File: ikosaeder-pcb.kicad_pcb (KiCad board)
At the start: 2 copper layers, 21.9 x 20.8 mm, 7 parts

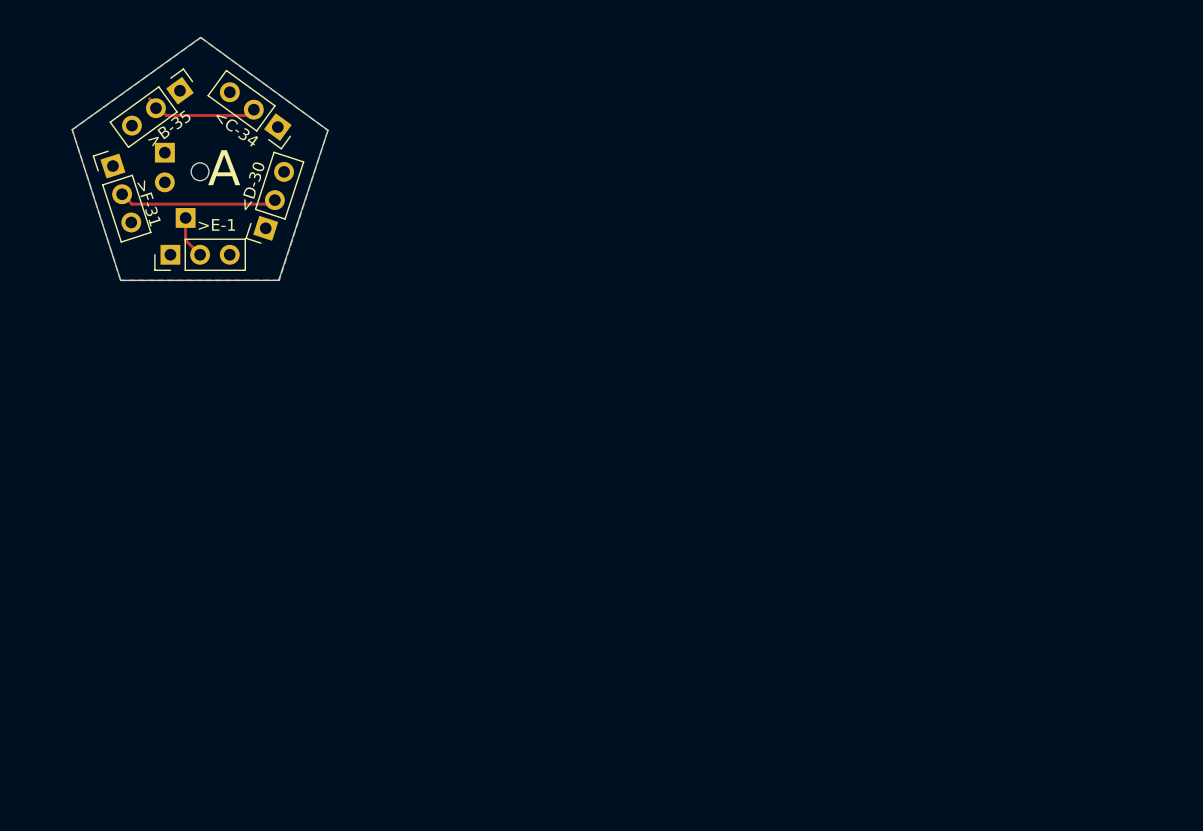
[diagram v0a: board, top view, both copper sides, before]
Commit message: Ikosaeder final
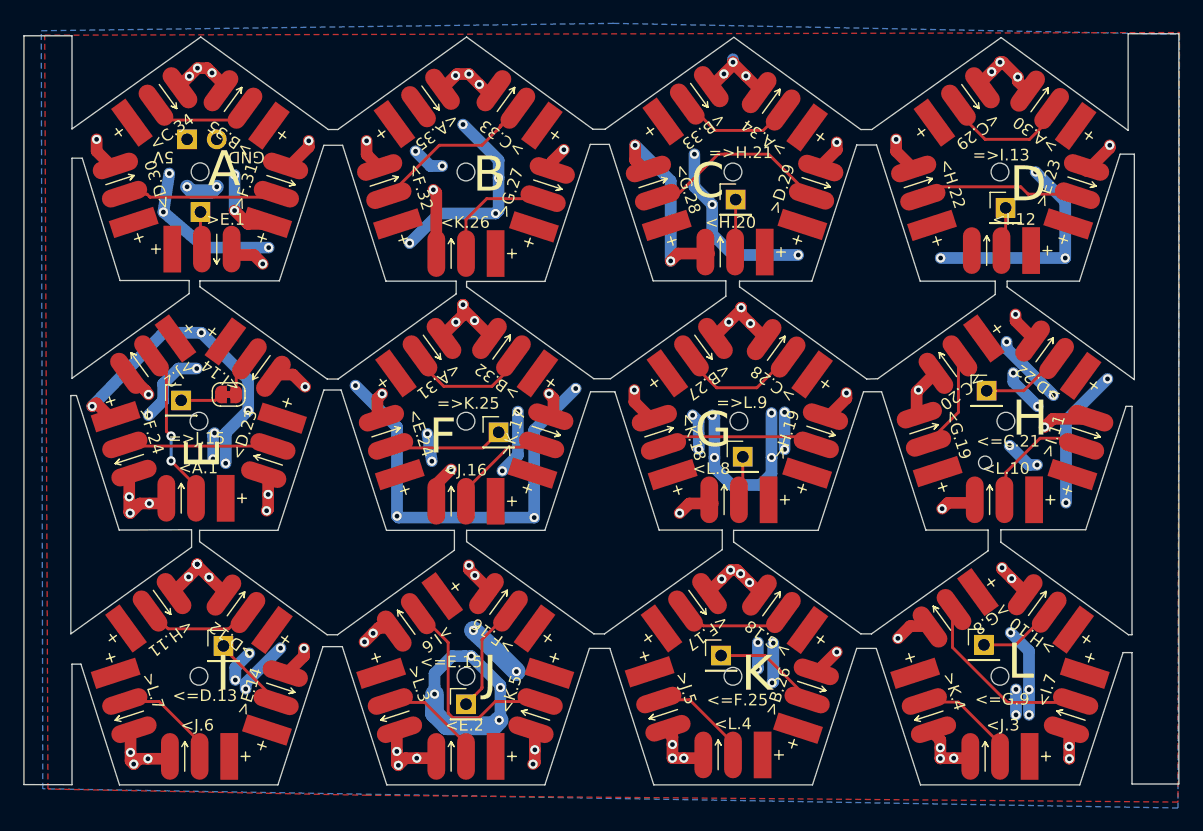
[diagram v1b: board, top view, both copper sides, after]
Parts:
- removed <C-34, <D-30: Conn_01x03_Female, Connector_PinSocket_2.54mm:PinSocket_1x03_P2.54mm_Vertical
- removed >B-35, >E-1, >F-31: Conn_01x03_Male, Connector_PinHeader_2.54mm:PinHeader_1x03_P2.54mm_Vertical
- added <=C.21: Conn_01x01_Female, Connector_PinHeader_2.54mm:PinHeader_1x01_P2.54mm_Vertical, F.Cu at (174.1, 105.6)
- added <=D.13: Conn_01x01_Female, Connector_PinHeader_2.54mm:PinHeader_1x01_P2.54mm_Vertical, F.Cu at (108.8, 127.4)
- added <=E.15: Conn_01x01_Female, Connector_PinHeader_2.54mm:PinHeader_1x01_P2.54mm_Vertical, F.Cu at (129.5, 132.4)
- added <=F.25: Conn_01x01_Female, Connector_PinHeader_2.54mm:PinHeader_1x01_P2.54mm_Vertical, F.Cu at (151.4, 128.3)
- added <=G.9: Conn_01x01_Female, Connector_PinHeader_2.54mm:PinHeader_1x01_P2.54mm_Vertical, F.Cu at (173.9, 127.4)
- added <A.1: LEDs_In, IkosaederFootprints:LED-Strip, F.Cu at (106.4, 114.8)
- added <A.31: LEDs_In, IkosaederFootprints:LED-Strip, F.Cu at (125.6, 102.6)
- added <A.35: LEDs_In, IkosaederFootprints:LED-Strip, F.Cu at (125.5, 81.3)
- added <B.27: LEDs_In, IkosaederFootprints:LED-Strip, F.Cu at (148.8, 102.6)
- added <B.33: LEDs_In, IkosaederFootprints:LED-Strip, F.Cu at (148.5, 81.1)
- added <C.29: LEDs_In, IkosaederFootprints:LED-Strip, F.Cu at (171.7, 81.2)
- added <C.34: LEDs_In, IkosaederFootprints:LED-Strip, F.Cu at (103.0, 81.2)
- added <D.23: LEDs_In, IkosaederFootprints:LED-Strip, F.Cu at (113.0, 110.4)
- added <D.30: LEDs_In, IkosaederFootprints:LED-Strip, F.Cu at (100.3, 88.8)
- added <E.2: LEDs_In, IkosaederFootprints:LED-Strip, F.Cu at (129.5, 136.9)
- added <E.24: LEDs_In, IkosaederFootprints:LED-Strip, F.Cu at (123.1, 110.4)
- added <F.17: LEDs_In, IkosaederFootprints:LED-Strip, F.Cu at (148.3, 124.5)
- added <F.32: LEDs_In, IkosaederFootprints:LED-Strip, F.Cu at (122.9, 88.9)
- added <G.19: LEDs_In, IkosaederFootprints:LED-Strip, F.Cu at (169.1, 110.1)
- added <G.28: LEDs_In, IkosaederFootprints:LED-Strip, F.Cu at (145.9, 89.0)
- added <H.11: LEDs_In, IkosaederFootprints:LED-Strip, F.Cu at (102.5, 124.5)
- added <H.20: LEDs_In, IkosaederFootprints:LED-Strip, F.Cu at (152.6, 93.7)
- added <H.22: LEDs_In, IkosaederFootprints:LED-Strip, F.Cu at (168.7, 89.0)
- added <I.12: LEDs_In, IkosaederFootprints:LED-Strip, F.Cu at (175.4, 93.6)
- added <I.14: LEDs_In, IkosaederFootprints:LED-Strip, F.Cu at (111.0, 102.9)
- added <I.7: LEDs_In, IkosaederFootprints:LED-Strip, F.Cu at (181.7, 132.2)
- added <J.16: LEDs_In, IkosaederFootprints:LED-Strip, F.Cu at (129.5, 115.1)
- added <J.3: LEDs_In, IkosaederFootprints:LED-Strip, F.Cu at (175.3, 136.9)
- added <J.6: LEDs_In, IkosaederFootprints:LED-Strip, F.Cu at (106.7, 136.9)
- added <K.18: LEDs_In, IkosaederFootprints:LED-Strip, F.Cu at (146.5, 110.4)
- added <K.26: LEDs_In, IkosaederFootprints:LED-Strip, F.Cu at (129.5, 93.9)
- added <K.5: LEDs_In, IkosaederFootprints:LED-Strip, F.Cu at (135.9, 132.2)
- added <L.10: LEDs_In, IkosaederFootprints:LED-Strip, F.Cu at (175.6, 114.9)
- added <L.4: LEDs_In, IkosaederFootprints:LED-Strip, F.Cu at (152.4, 136.8)
- added <L.8: LEDs_In, IkosaederFootprints:LED-Strip, F.Cu at (152.9, 114.9)
- added =>H.21: Conn_01x01_Male, Connector_PinHeader_2.54mm:PinHeader_1x01_P2.54mm_Vertical, F.Cu at (152.6, 89.2)
- added =>I.13: Conn_01x01_Male, Connector_PinHeader_2.54mm:PinHeader_1x01_P2.54mm_Vertical, F.Cu at (175.7, 89.9)
- added =>J.15: Conn_01x01_Male, Connector_PinHeader_2.54mm:PinHeader_1x01_P2.54mm_Vertical, F.Cu at (105.2, 106.4)
- added =>K.25: Conn_01x01_Male, Connector_PinHeader_2.54mm:PinHeader_1x01_P2.54mm_Vertical, F.Cu at (132.3, 109.2)
- added =>L.9: Conn_01x01_Male, Connector_PinHeader_2.54mm:PinHeader_1x01_P2.54mm_Vertical, F.Cu at (153.2, 111.3)
- added >A.30: LEDs_Out, IkosaederFootprints:LED-Strip, F.Cu at (179.7, 81.4)
- added >A.34: LEDs_Out, IkosaederFootprints:LED-Strip, F.Cu at (156.7, 81.6)
- added >B.26: LEDs_Out, IkosaederFootprints:LED-Strip, F.Cu at (158.8, 132.1)
- added >B.32: LEDs_Out, IkosaederFootprints:LED-Strip, F.Cu at (133.6, 102.6)
- added >B.35: LEDs_Out, IkosaederFootprints:LED-Strip, F.Cu at (110.6, 81.4)
- added >C.20: LEDs_Out, IkosaederFootprints:LED-Strip, F.Cu at (171.8, 102.6)
- added >C.28: LEDs_Out, IkosaederFootprints:LED-Strip, F.Cu at (157.1, 102.7)
- added >C.33: LEDs_Out, IkosaederFootprints:LED-Strip, F.Cu at (134.0, 81.4)
- added >D.12: LEDs_Out, IkosaederFootprints:LED-Strip, F.Cu at (110.9, 124.6)
- added >D.22: LEDs_Out, IkosaederFootprints:LED-Strip, F.Cu at (180.1, 102.8)
- added >D.29: LEDs_Out, IkosaederFootprints:LED-Strip, F.Cu at (159.1, 88.9)
- added >E.1: LEDs_Out, IkosaederFootprints:LED-Strip, F.Cu at (106.9, 93.5)
- added >E.14: LEDs_Out, IkosaederFootprints:LED-Strip, F.Cu at (113.3, 132.2)
- added >E.23: LEDs_Out, IkosaederFootprints:LED-Strip, F.Cu at (181.9, 88.9)
- added >F.16: LEDs_Out, IkosaederFootprints:LED-Strip, F.Cu at (133.3, 124.5)
- added >F.24: LEDs_Out, IkosaederFootprints:LED-Strip, F.Cu at (100.3, 110.2)
- added >F.31: LEDs_Out, IkosaederFootprints:LED-Strip, F.Cu at (113.3, 88.8)
- added >G.18: LEDs_Out, IkosaederFootprints:LED-Strip, F.Cu at (156.7, 124.6)
- added >G.27: LEDs_Out, IkosaederFootprints:LED-Strip, F.Cu at (136.1, 89.2)
- added >G.8: LEDs_Out, IkosaederFootprints:LED-Strip, F.Cu at (171.3, 124.3)
- added >H.10: LEDs_Out, IkosaederFootprints:LED-Strip, F.Cu at (179.5, 124.6)
- added >H.19: LEDs_Out, IkosaederFootprints:LED-Strip, F.Cu at (159.5, 110.2)
- added >I.11: LEDs_Out, IkosaederFootprints:LED-Strip, F.Cu at (182.2, 110.4)
- added >I.6: LEDs_Out, IkosaederFootprints:LED-Strip, F.Cu at (125.5, 124.7)
- added >J.2: LEDs_Out, IkosaederFootprints:LED-Strip, F.Cu at (102.6, 102.6)
- added >J.5: LEDs_Out, IkosaederFootprints:LED-Strip, F.Cu at (146.1, 132.1)
- added >K.17: LEDs_Out, IkosaederFootprints:LED-Strip, F.Cu at (136.0, 110.2)
- added >K.4: LEDs_Out, IkosaederFootprints:LED-Strip, F.Cu at (168.8, 132.2)
- added >L.3: LEDs_Out, IkosaederFootprints:LED-Strip, F.Cu at (123.1, 132.2)
- added >L.7: LEDs_Out, IkosaederFootprints:LED-Strip, F.Cu at (100.3, 132.2)
- added G***: LOGO, LOGO, B.Cu at (175.3, 123.9)
- added G***: LOGO, LOGO, B.Cu at (152.4, 87.1)
- added G***: LOGO, LOGO, B.Cu at (132.8, 91.9)
- added G***: LOGO, LOGO, B.Cu at (152.5, 130.2)
- added G***: LOGO, LOGO, B.Cu at (135.4, 128.2)
- added G***: LOGO, LOGO, B.Cu at (106.7, 124.0)
- added G***: LOGO, LOGO, B.Cu at (110.3, 113.4)
- added G***: LOGO, LOGO, B.Cu at (125.8, 113.8)
- added G***: LOGO, LOGO, B.Cu at (153.1, 102.0)
- added G***: LOGO, LOGO, B.Cu at (170.0, 106.5)
- added G***: LOGO, LOGO, B.Cu at (179.4, 92.3)
- added JP1: SolderJumper_2_Bridged, Jumper:SolderJumper-2_P1.3mm_Bridged_RoundedPad1.0x1.5mm, F.Cu at (109.2, 105.9)
- moved Power1 2.22 mm to (105.7, 84.1), turned to -90 degrees
- moved DIN1 1.37 mm to (106.8, 90.3)
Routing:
- net +5V: track 0.00 -> 254.8 mm, vias 0 -> 70
- net GND: track 0.00 -> 190.5 mm, vias 0 -> 79
- net Net-(<K.5-Pad2): track 0.00 -> 18.9 mm
- net Net-(<G.28-Pad2): track 0.00 -> 16.5 mm
- net Net-(<I.7-Pad2): track 0.00 -> 16.0 mm
- net Net-(<F.32-Pad2): track 0.00 -> 16.0 mm
- net Net-(<D.30-Pad2): track 0.00 -> 15.9 mm
- net Net-(<H.22-Pad2): track 0.00 -> 14.9 mm
- net Net-(<A.1-Pad2): track 0.00 -> 14.5 mm, vias 0 -> 2
- net Net-(<K.18-Pad2): track 0.00 -> 14.2 mm
- net Net-(<D-30-Pad2): track 13.6 -> 0.00 mm
- net Net-(<D.23-Pad2): track 0.00 -> 13.5 mm
- net Net-(<C.29-Pad2): track 0.00 -> 11.6 mm
- net Net-(<F.17-Pad2): track 0.00 -> 11.5 mm
- net Net-(<A.31-Pad2): track 0.00 -> 11.5 mm
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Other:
- board size 21.9 x 20.8 mm -> 98.9 x 64.3 mm
- net class 5V added: clearance 0.2, trace_width 1, via_dia 0.8, via_drill 0.4
- net class GND added: clearance 0.2, trace_width 1, via_dia 0.8, via_drill 0.4
- board text added: "April 2020"
- board text added: "B"
- board text added: "By BeFaFl"
- board text added: "C"
- board text added: "D"
- board text added: "Designed in Zurich"
- board text added: "E"
- board text added: "EAST"
- board text added: "F"
- board text added: "FIN."
- board text added: "G"
- board text added: "H"
- board text added: "HICKEN!"
- board text added: "I"
- board text added: "J"
- board text added: "JLCJLCJLCJLC"
- board text added: "June-ish 2020"
- board text added: "K"
- board text added: "L"
- board text added: "LE"
- board text added: "Mind the"
- board text added: "NORTH"
- board text added: "NORTHWEST"
- board text added: "Order Nr."
- board text added: "SOUTH"
- board text added: "This is me!"
- board text added: "V1.0"
- board text added: "eep the GND plane"
- board text added: "github.com/BeFaFl"
- board text added: "leen"
